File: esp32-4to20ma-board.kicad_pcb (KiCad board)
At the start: 2 copper layers, 40 x 61 mm, 59 parts, among them J1 USB-C Receptacle, J2 4-20mA Loop, Q1 BCP53-16, Q2 MMBT5401, Q3 AO3401A, Q4 2N7002, SW1 RESET, SW2 BOOT, U1 ESP32-S3-WROOM-1U-N4, U3 INA226AIDGSR, U4 AP2112K-3.3, U5 MT3608

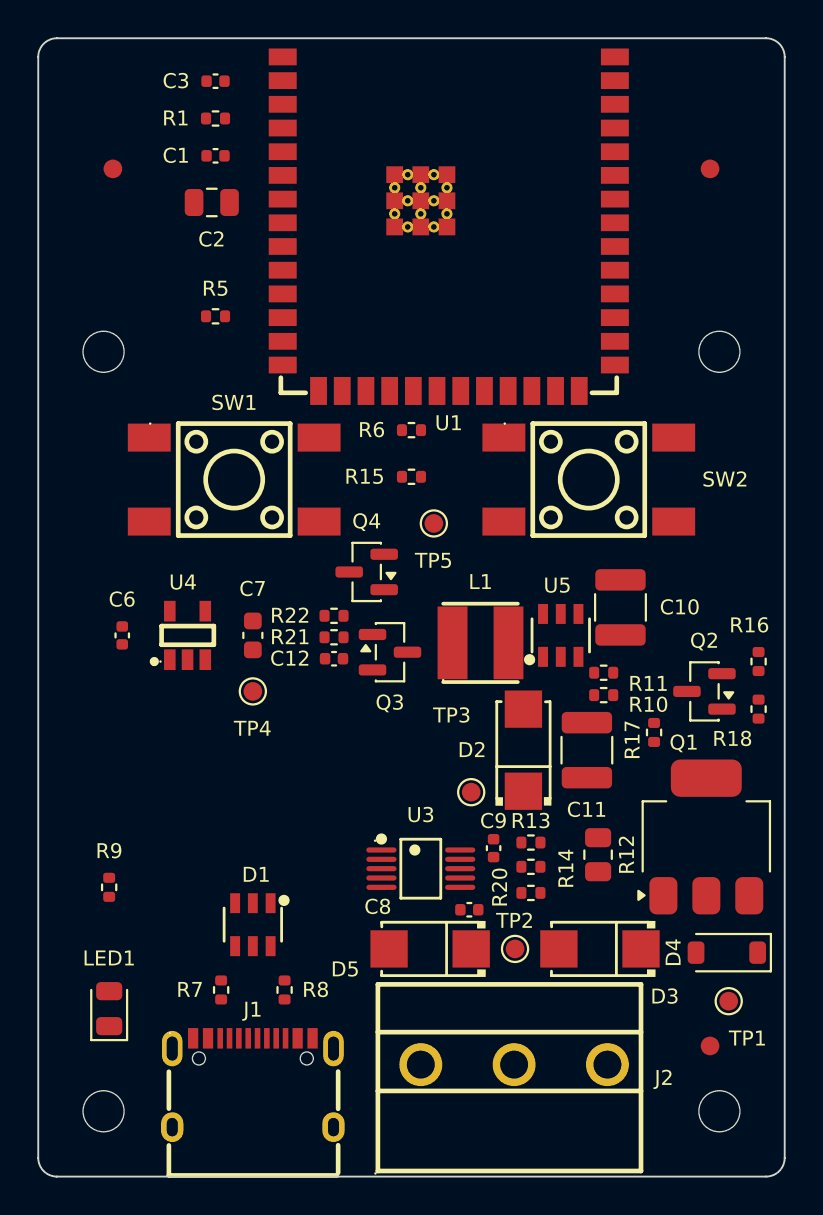
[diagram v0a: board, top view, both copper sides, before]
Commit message: docs: describe the firmware as a published remote package
Co-Authored-By: Claude Opus 5 <noreply@anthropic.com>
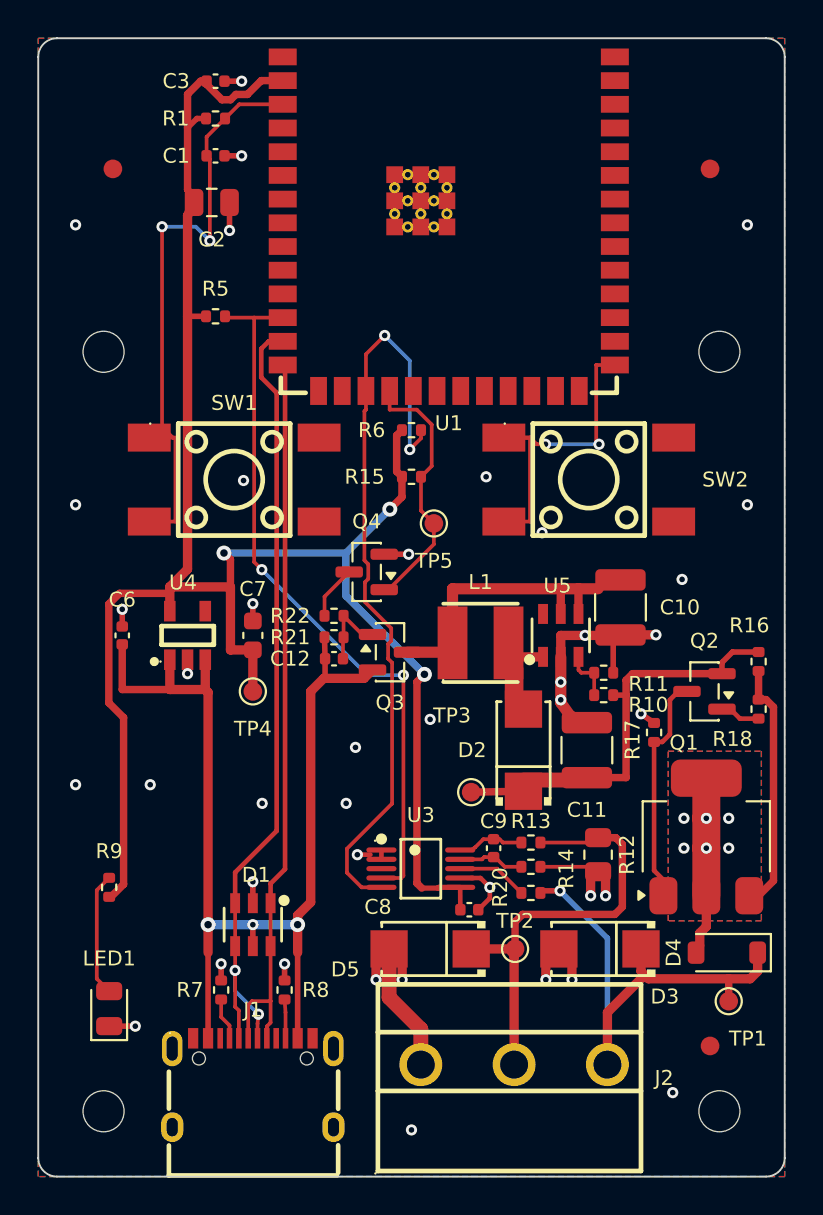
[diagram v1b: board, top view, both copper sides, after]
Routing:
- net +3V3: track 0.00 -> 107.5 mm, vias 0 -> 3
- net +5V: track 0.00 -> 59.6 mm, vias 0 -> 3
- net /USB_N: track 0.00 -> 43.8 mm, vias 0 -> 2
- net /I2C_SCL: track 0.00 -> 41.3 mm, vias 0 -> 2
- net GND: track 0.00 -> 39.8 mm, vias 0 -> 40
- net /USB_P: track 0.00 -> 39.6 mm
- net /I2C_SDA: track 0.00 -> 38.7 mm, vias 0 -> 2
- net /EN: track 0.00 -> 32.2 mm, vias 0 -> 2
- net /LOOP_V: track 0.00 -> 27.2 mm, vias 0 -> 1
- net /LOOP_RTN: track 0.00 -> 23.3 mm
- net +24V: track 0.00 -> 21.1 mm
- net /IO0: track 0.00 -> 17.9 mm, vias 0 -> 2
- net /MT_EN: track 0.00 -> 14.2 mm
- net /LOOP_SNS: track 0.00 -> 13.4 mm
- net /VIN_SW: track 0.00 -> 13.4 mm
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- added copper zone on B.Cu, net /LOOP_C
- added copper zone on F.Cu, net /LOOP_C
- added copper zone on B.Cu, net GND
- added copper zone on F.Cu, net GND
